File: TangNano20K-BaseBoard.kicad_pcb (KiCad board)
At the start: 2 copper layers, 100 x 100 mm, 48 parts, among them J1 Conn_01x20_Socket, J2 Conn_01x20_Socket, J3 Conn_02x06_Odd_Even, Q1 PN2222A, Q2 PN2222A, Q3 PN2222A, Q4 PN2222A, SW1 SW_SPDT_321, SW2 SW_SPDT_321, SW3 SW_SPDT_321, SW4 SW_SPDT_321, SW5 SW_SPDT_321, U1 CC56-12EWA, U2 SSD1306

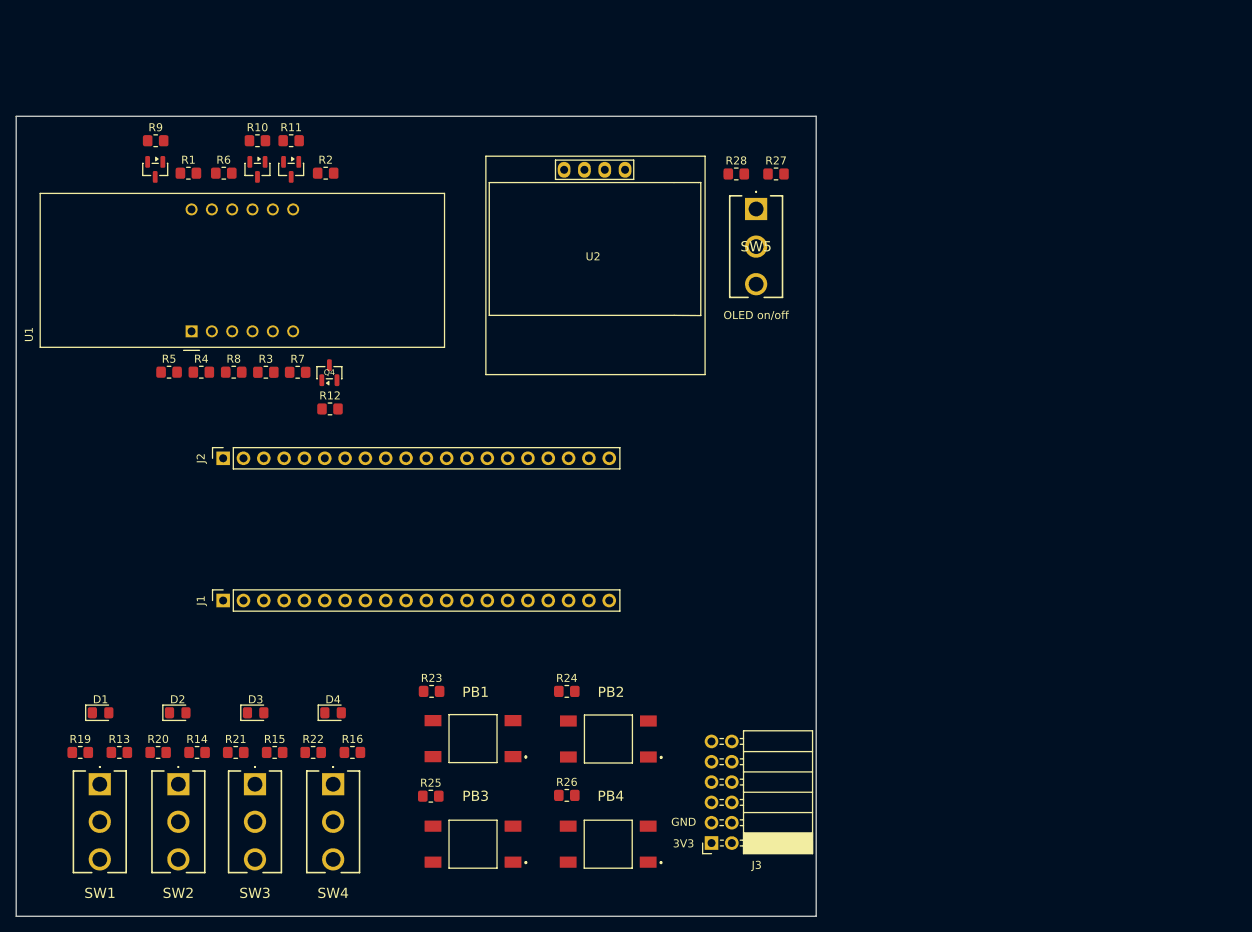
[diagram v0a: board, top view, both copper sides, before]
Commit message: Update pcb
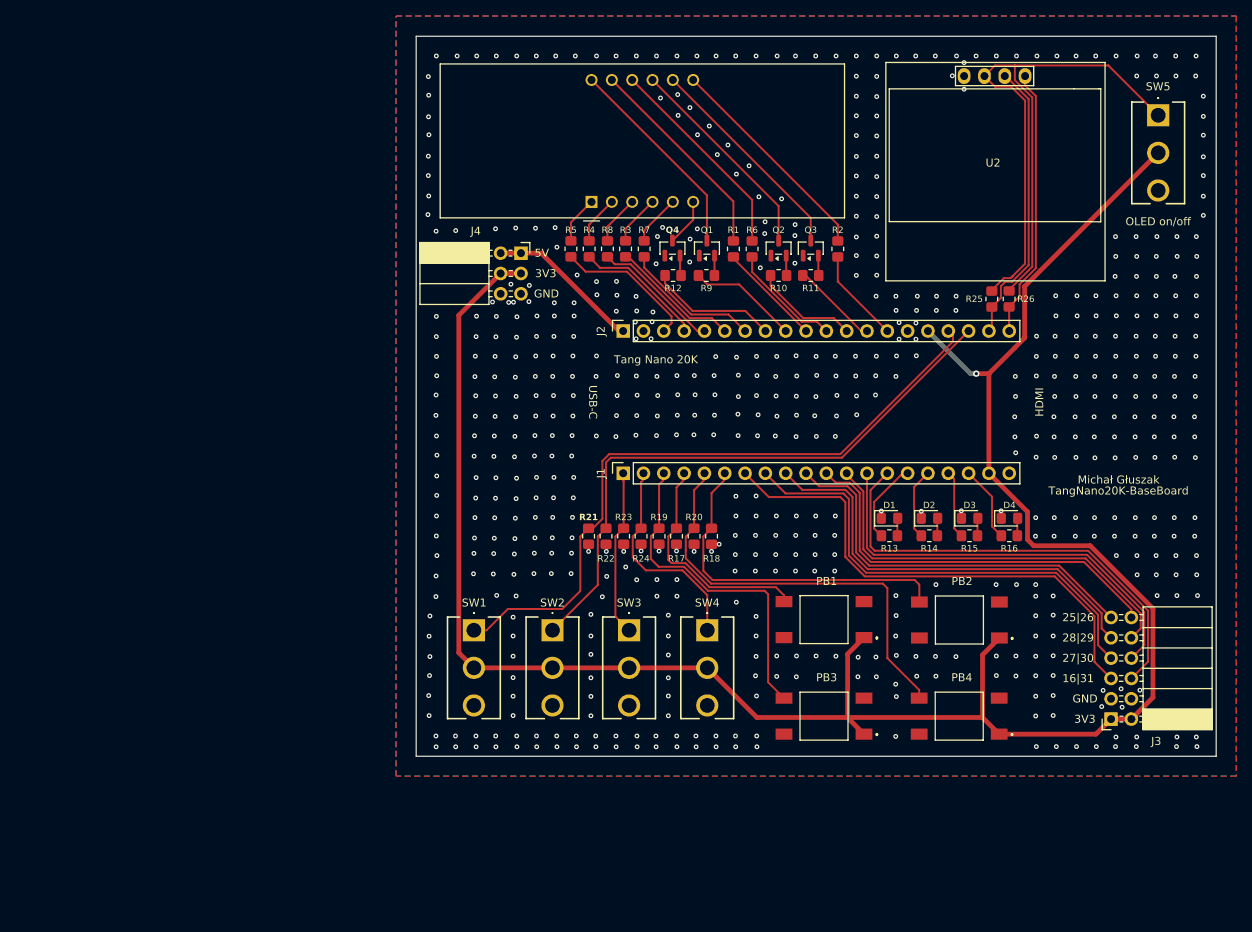
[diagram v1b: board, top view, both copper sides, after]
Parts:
- added J4: Conn_02x03_Odd, Connector_PinSocket_2.54mm:PinSocket_2x03_P2.54mm_Horizontal, F.Cu at (213.1, 87.1)
- moved D1 101.6 mm to (259.2, 120.3)
- moved R13 100.0 mm to (259.2, 122.4)
- moved D2 97.1 mm to (264.2, 120.3)
- moved R14 95.5 mm to (264.1, 122.4)
- moved D3 92.5 mm to (269.2, 120.3)
- moved R15 91.0 mm to (269.2, 122.4)
- moved D4 88.0 mm to (274.2, 120.3)
- moved R16 86.5 mm to (274.1, 122.4)
- moved R9 70.9 mm to (236.3, 89.9), turned to 180 degrees
- moved Q1 69.7 mm to (236.3, 86.5), turned to 90 degrees
- moved R21 69.0 mm to (221.6, 122.5), turned to 90 degrees
- moved R1 68.8 mm to (239.7, 86.6), turned to 90 degrees
- moved R10 67.3 mm to (245.3, 89.9), turned to 180 degrees
- moved R11 67.1 mm to (249.3, 89.9), turned to 180 degrees
- moved R6 66.7 mm to (242.0, 86.6), turned to 90 degrees
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- renumbered R23 to R17, R24 to R18, R25 to R19, R26 to R20, R19 to R21, R20 to R22, R21 to R23, R22 to R24, R27 to R25, R28 to R26
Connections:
- J3 pad 10: /30 -> /29
- J3 pad 11: /72 -> /25
- J3 pad 12: /31 -> /26
- J3 pad 5: /15 -> /16
- J3 pad 6: /26 -> /31
- J3 pad 7: /16 -> /27
- J3 pad 8: /29 -> /30
- J3 pad 9: /71 -> /28
- PB1 pad 4: /77 -> /85
- PB2 pad 4: /27 -> /15
- PB3 pad 4: /28 -> /75
- PB4 pad 4: /25 -> /77
- R17 pad 2: /77 -> /85
- R18 pad 2: /27 -> /15
- R19 pad 2: /28 -> /75
- R20 pad 2: /25 -> /77
- R21 pad 2: /73 -> /72
- R22 pad 2: /74 -> /71
- R23 pad 2: /75 -> /73
- R24 pad 2: /85 -> /74
- SW1 pad 1: /73 -> /72
- SW2 pad 1: /74 -> /71
- SW3 pad 1: /75 -> /73
- SW4 pad 1: /85 -> /74
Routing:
- net +3V3: track 0.00 -> 268.9 mm, vias 0 -> 1
- net Net-(SW5-C): track 0.00 -> 87.7 mm
- net /72: track 0.00 -> 84.6 mm
- net /71: track 0.00 -> 75.9 mm
- net /16: track 0.00 -> 63.7 mm
- net /27: track 0.00 -> 59.1 mm
- net /31: track 0.00 -> 57.4 mm
- net /28: track 0.00 -> 54.5 mm
- net /30: track 0.00 -> 53.8 mm
- net /77: track 0.00 -> 52.9 mm
- net /29: track 0.00 -> 51.9 mm
- net /26: track 0.00 -> 50.5 mm
- net /25: track 0.00 -> 49.8 mm
- net /15: track 0.00 -> 42.3 mm
- net /75: track 0.00 -> 40.8 mm
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- added copper zone on B.Cu, net GND
- added copper zone on F.Cu, net GND
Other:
- board size 100 x 100 mm -> 100 x 90 mm
- board text added: "16|31"
- board text added: "25|26"
- board text added: "27|30"
- board text added: "28|29"
- board text added: "5V"
- board text added: "HDMI"
- board text added: "Michał Głuszak"
- board text added: "Tang Nano 20K"
- board text added: "TangNano20K-BaseBoard"
- board text added: "USB-C"
- board text removed: "Q4"
